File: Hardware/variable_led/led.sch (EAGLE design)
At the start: 12 parts

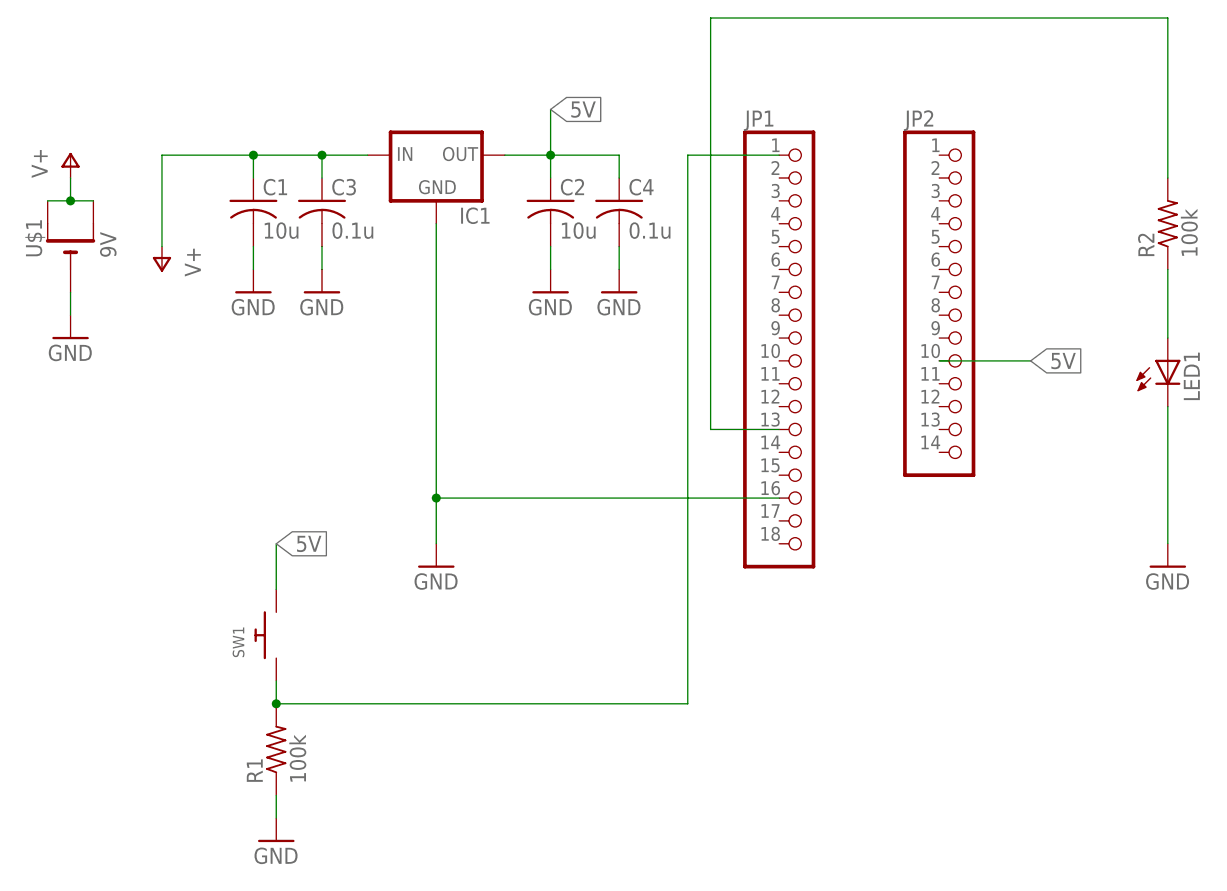
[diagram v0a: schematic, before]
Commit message: Updated PCB based on feedback
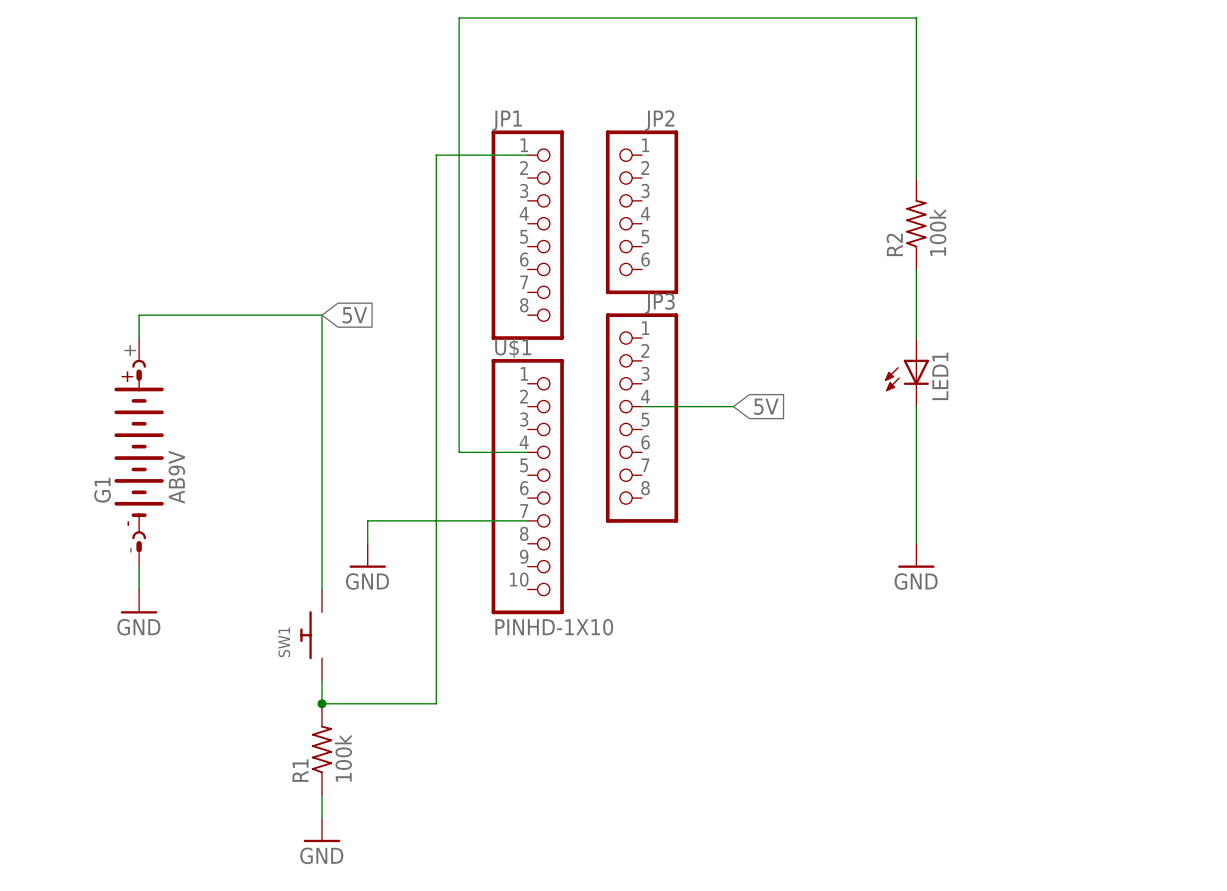
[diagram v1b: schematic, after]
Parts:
- removed C1, C2: 10u, adafruit:C-USC0805
- removed C3, C4: 0.1u, adafruit:C-USC0805
- removed IC1: (no value), v-reg:78XXL
- added G1: AB9V, battery:AB9V
- added JP3: (no value), adafruit:PINHD-1X8BIG
- JP1: device adafruit:PINHD-1X18 -> adafruit:PINHD-1X8BIG
- JP2: device adafruit:PINHD-1X14 -> adafruit:PINHD-1X6B
- U$1: value 9V -> PINHD-1X10; device adafruit:CR1220SMT -> adafruit:PINHD-1X10
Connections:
- removed net V+: C1.1, C3.1, IC1.IN, U$1.+, U$1.+1
- net 5V: now also G1.+, JP3.4; no longer C2.1, C4.1, IC1.OUT, JP2.10
- net GND: now also G1.-, U$1.7; no longer C1.2, C2.2, C3.2, C4.2, IC1.GND, JP1.16, U$1.-
- net N$2: now also U$1.4; no longer JP1.13
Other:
- moved on the sheet: LED1, R1, R2, SW1
